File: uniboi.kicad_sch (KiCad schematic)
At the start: 18 parts, among them J1 DX07S016JA3R1500, J4 SW_pads, SW1 SW_Push, SW2 SW_SPDT, U1 XC6206P332MR, U2 SRV05-4, U3 STM32G0B1CBT6

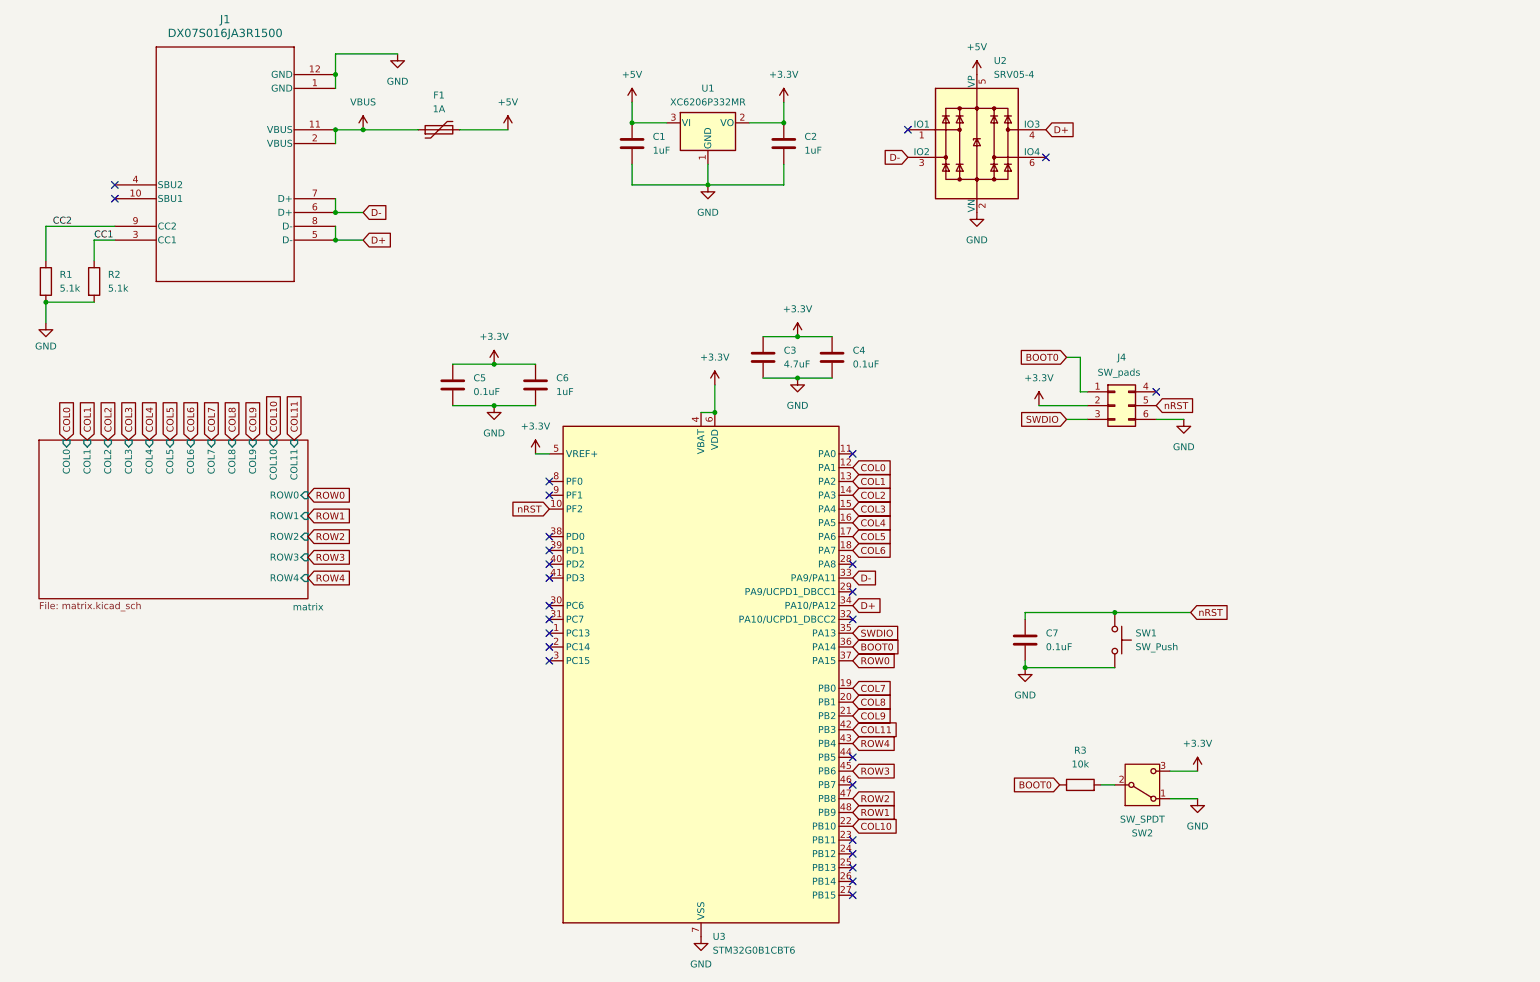
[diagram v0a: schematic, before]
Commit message: clean up and final touches
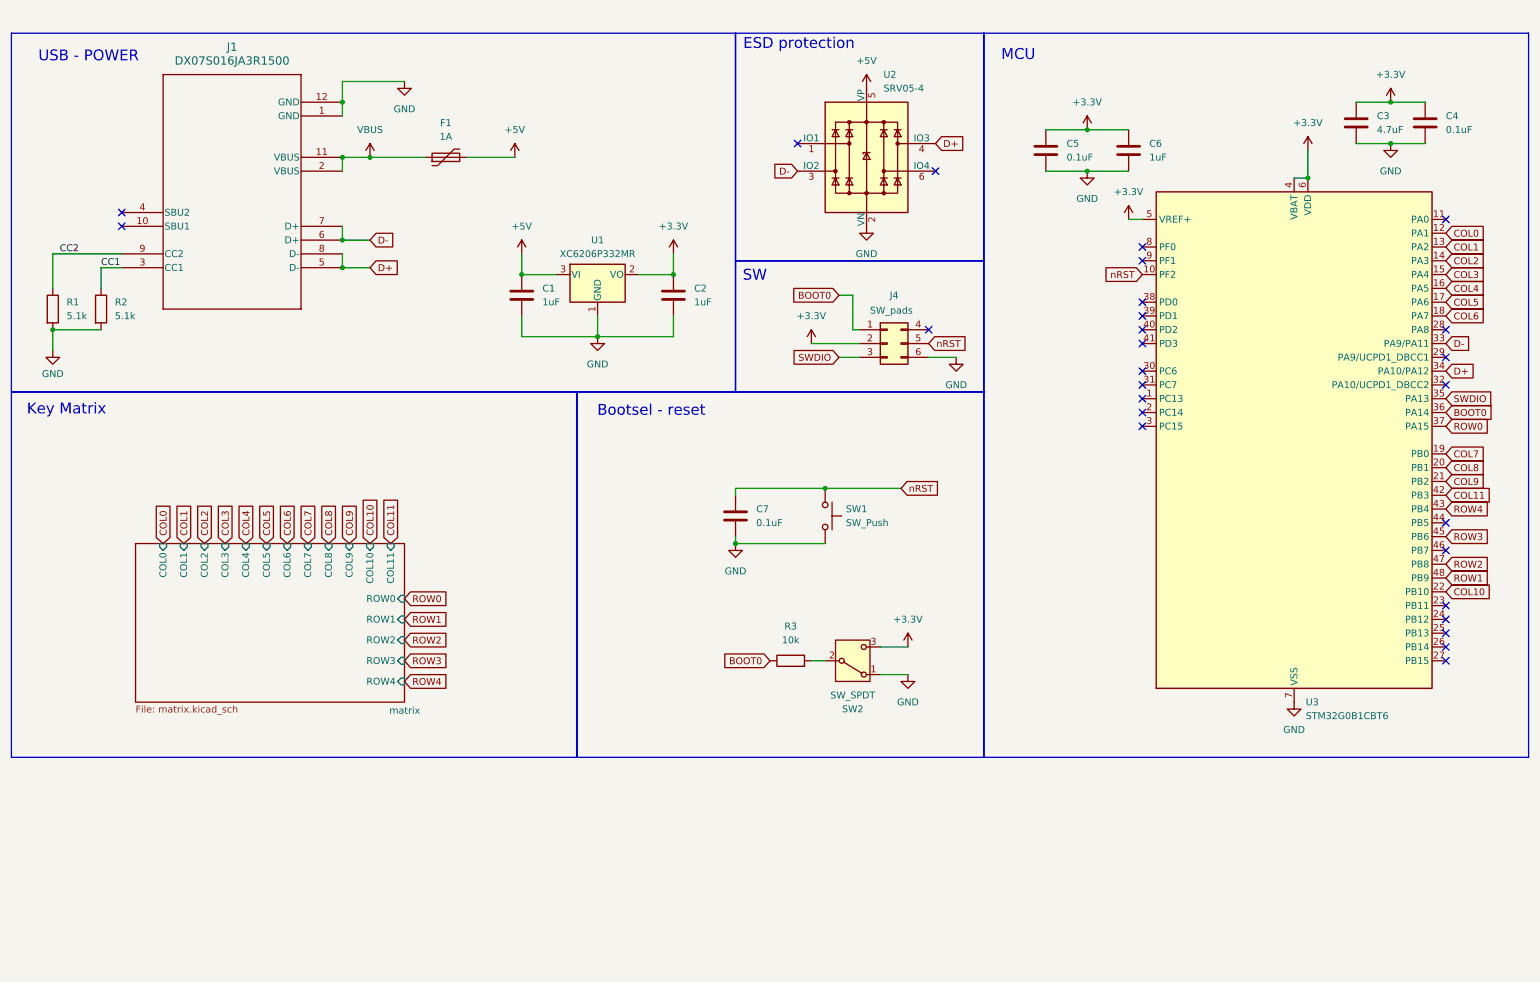
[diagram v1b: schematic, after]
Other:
- note added: "Bootsel - reset"
- note added: "ESD protection"
- note added: "Key Matrix"
- note added: "MCU"
- note added: "SW"
- note added: "USB - POWER"
- moved on the sheet: C1, C2, C3, C4, C5, C6, C7, F1, J1, J4, R1, R2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

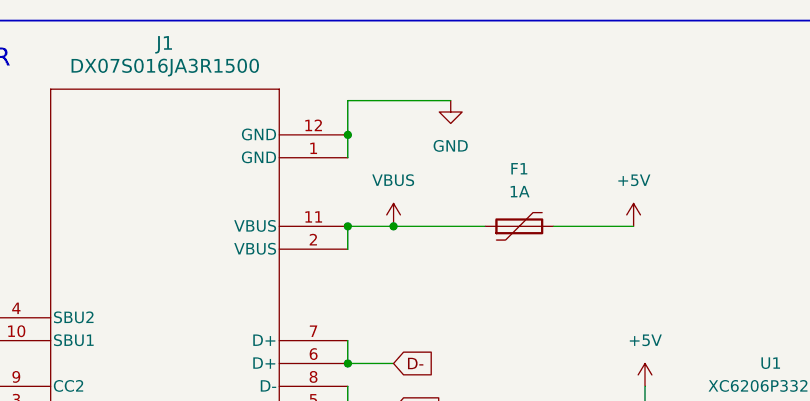
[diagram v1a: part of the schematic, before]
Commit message: clean up and final touches
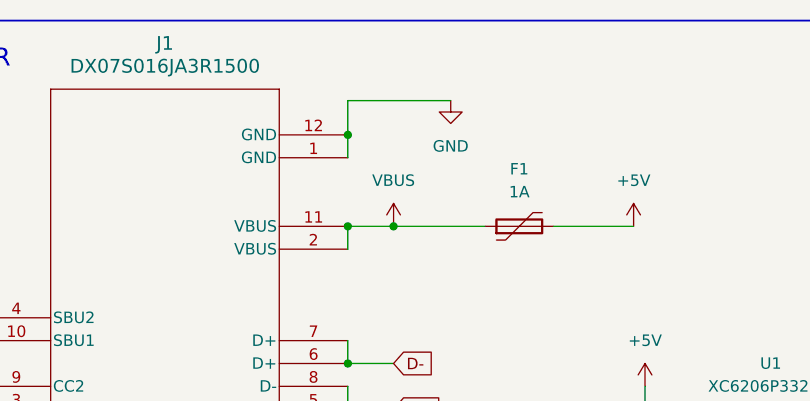
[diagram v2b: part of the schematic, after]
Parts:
- J4: footprint Connector:Tag-Connect_TC2030-IDC-NL_2x03_P1.27mm_Vertical -> connector:Tag-Connect_TC2030-IDC-NL_2x03_P1.27mm_Vertical
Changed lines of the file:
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@@
 	)
 	(junction
-		(at 77.47 34.29)
-		(diameter 0)
-		(color 0 0 0 0)
-	)
-	(junction
 		(at 24.13 76.2)
 		(diameter 0)
@@
 	)
 	(junction
+		(at 77.47 34.29)
+		(diameter 0)
+		(color 0 0 0 0)
+	)
+	(junction
 		(at 124.46 77.47)
 		(diameter 0)
@@
 	(wire
 		(pts
-			(xy 77.47 30.48) (xy 77.47 34.29)
-		)
-		(stroke
-			(width 0)
-			(type default)
-		)
-	)
-	(wire
-		(pts
 			(xy 149.86 115.57) (xy 166.37 115.57)
 		)
@@
 	(wire
 		(pts
-			(xy 77.47 34.29) (xy 77.47 36.83)
+			(xy 77.47 62.23) (xy 77.47 64.77)
 		)
 		(stroke
@@
 	(wire
 		(pts
-			(xy 77.47 62.23) (xy 77.47 64.77)
+			(xy 100.33 44.45) (xy 109.22 44.45)
 		)
 		(stroke
@@
 	(wire
 		(pts
-			(xy 100.33 44.45) (xy 109.22 44.45)
+			(xy 132.08 66.04) (xy 138.43 66.04)
 		)
 		(stroke
@@
 	(wire
 		(pts
-			(xy 132.08 66.04) (xy 138.43 66.04)
+			(xy 77.47 30.48) (xy 88.9 30.48)
 		)
 		(stroke
@@
 	(wire
 		(pts
-			(xy 77.47 30.48) (xy 88.9 30.48)
+			(xy 110.49 73.66) (xy 110.49 77.47)
 		)
 		(stroke
@@
 	(wire
 		(pts
-			(xy 110.49 73.66) (xy 110.49 77.47)
+			(xy 33.02 64.77) (xy 36.83 64.77)
 		)
 		(stroke
@@
 	(wire
 		(pts
-			(xy 33.02 64.77) (xy 36.83 64.77)
+			(xy 163.83 78.74) (xy 172.72 78.74)
 		)
 		(stroke
@@
 	(wire
 		(pts
-			(xy 163.83 78.74) (xy 172.72 78.74)
+			(xy 176.53 139.7) (xy 181.61 139.7)
 		)
 		(stroke
@@
 	(wire
 		(pts
-			(xy 176.53 139.7) (xy 181.61 139.7)
+			(xy 77.47 34.29) (xy 77.47 36.83)
 		)
 		(stroke
@@
 	(wire
 		(pts
+			(xy 77.47 34.29) (xy 77.47 30.48)
+		)
+		(stroke
+			(width 0)
+			(type default)
+		)
+	)
+	(wire
+		(pts
 			(xy 138.43 62.23) (xy 138.43 66.04)
 		)
@@
 	)
 	(symbol
-		(lib_id "power:GND")
-		(at 88.9 30.48 0)
-		(unit 1)
-		(exclude_from_sim no)
-		(in_bom yes)
-		(on_board yes)
-		(dnp no)
-		(fields_autoplaced yes)
-		(property "Reference" "#PWR01"
-			(at 88.9 36.83 0)
-			(effects
-				(font
-					(size 1.27 1.27)
-				)
-				(hide yes)
-			)
-		)
-		(property "Value" "GND"
-			(at 88.9 35.56 0)
-			(effects
-				(font
-					(size 1.27 1.27)
-				)
-			)
-		)
-		(property "Footprint" ""
-			(at 88.9 30.48 0)
-			(effects
-				(font
-					(size 1.27 1.27)
-				)
-				(hide yes)
-			)
-		)
-		(property "Datasheet" ""
-			(at 88.9 30.48 0)
-			(effects
-				(font
-					(size 1.27 1.27)
-				)
-				(hide yes)
-			)
-		)
-		(property "Description" "Power symbol creates a global label with name \"GND\" , ground"
-			(at 88.9 30.48 0)
-			(effects
-				(font
-					(size 1.27 1.27)
-				)
-				(hide yes)
-			)
-		)
-		(pin "1"
-		)
-		(instances
-			(project ""
-				(path "/68edf1f0-3df8-4c26-9976-9a41f0a4fe75"
-					(reference "#PWR01")
-					(unit 1)
-				)
-			)
-		)
-	)
-	(symbol
 		(lib_id "power:+5V")
 		(at 110.49 62.23 0)
@@
 	)
 	(symbol
+		(lib_id "power:GND")
+		(at 88.9 30.48 0)
+		(mirror y)
+		(unit 1)
+		(exclude_from_sim no)
+		(in_bom yes)
+		(on_board yes)
+		(dnp no)
+		(property "Reference" "#PWR023"
+			(at 88.9 36.83 0)
+			(effects
+				(font
+					(size 1.27 1.27)
+				)
+				(hide yes)
+			)
+		)
+		(property "Value" "GND"
+			(at 88.9 35.56 0)
+			(effects
+				(font
+					(size 1.27 1.27)
+				)
+			)
+		)
+		(property "Footprint" ""
+			(at 88.9 30.48 0)
+			(effects
+				(font
+					(size 1.27 1.27)
+				)
+				(hide yes)
+			)
+		)
+		(property "Datasheet" ""
+			(at 88.9 30.48 0)
+			(effects
+				(font
+					(size 1.27 1.27)
+				)
+				(hide yes)
+			)
+		)
+		(property "Description" "Power symbol creates a global label with name \"GND\" , ground"
+			(at 88.9 30.48 0)
+			(effects
+				(font
+					(size 1.27 1.27)
+				)
+				(hide yes)
+			)
+		)
+		(pin "1"
+		)
+		(instances
+			(project "uniboi"
+				(path "/68edf1f0-3df8-4c26-9976-9a41f0a4fe75"
+					(reference "#PWR023")
+					(unit 1)
+				)
+			)
+		)
+	)
+	(symbol
 		(lib_id "Regulator_Linear:XC6206PxxxMR")
 		(at 124.46 66.04 0)
@@
 			)
 		)
-		(property "Footprint" "Connector:Tag-Connect_TC2030-IDC-NL_2x03_P1.27mm_Vertical"
+		(property "Footprint" "connector:Tag-Connect_TC2030-IDC-NL_2x03_P1.27mm_Vertical"
 			(at 177.8 78.74 0)
 			(effects
